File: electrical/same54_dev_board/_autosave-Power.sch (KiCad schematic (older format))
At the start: 1 part

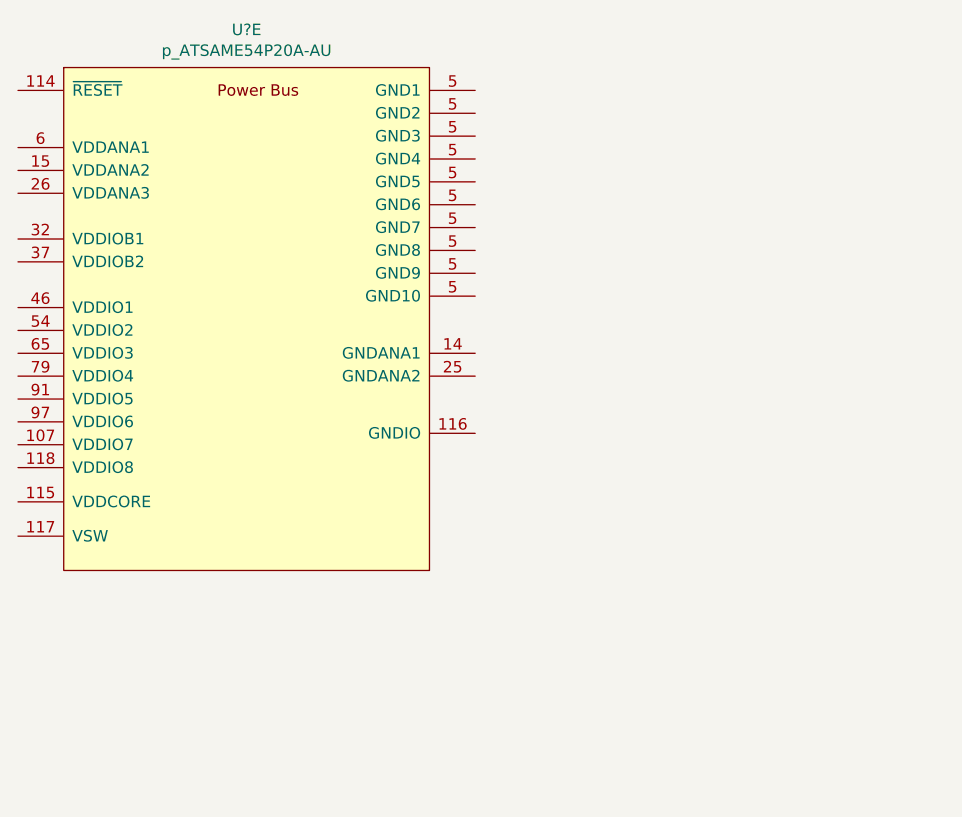
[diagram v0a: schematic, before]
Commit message: made some connections, creating firmware base from asf4
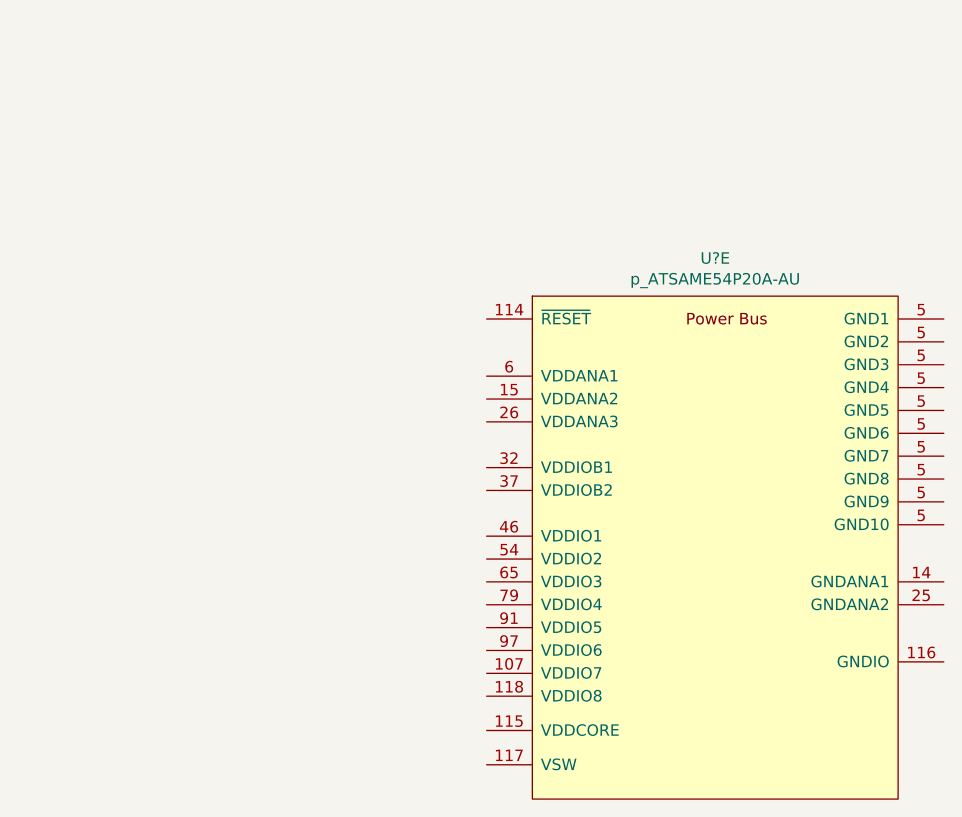
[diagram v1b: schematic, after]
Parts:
- removed U?: p_ATSAME54P20A-AU, symbol p_ATSAME54P20A-AU:p_ATSAME54P20A-AU
- added U?: p_ATSAME54P20A-AU, symbol p_ATSAME54P20A-AU:p_ATSAME54P20A-AU
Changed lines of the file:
@@
 $Descr A4 11693 8268
 encoding utf-8
-Sheet 2 2
+Sheet 2 4
 Title ""
 Date ""
@@
 $Comp
 L p_ATSAME54P20A-AU:p_ATSAME54P20A-AU U?
-U 5 1 5E7A11E1
-P 2750 2300
-F 0 "U?" H 2750 3215 50  0000 C CNN
-F 1 "p_ATSAME54P20A-AU" H 2750 3124 50  0000 C CNN
-F 2 "" H 1550 3550 50  0001 C CNN
-F 3 "" H 1550 3550 50  0001 C CNN
-	5    2750 2300
+U 5 1 5E84F3B3
+P 4800 3300
+F 0 "U?" H 4800 4215 50  0000 C CNN
+F 1 "p_ATSAME54P20A-AU" H 4800 4124 50  0000 C CNN
+F 2 "" H 3600 4550 50  0001 C CNN
+F 3 "" H 3600 4550 50  0001 C CNN
+	5    4800 3300
 	1    0    0    -1
 $EndComp
